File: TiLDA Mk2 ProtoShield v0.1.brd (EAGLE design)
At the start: 67.9 x 100 mm, 104 parts

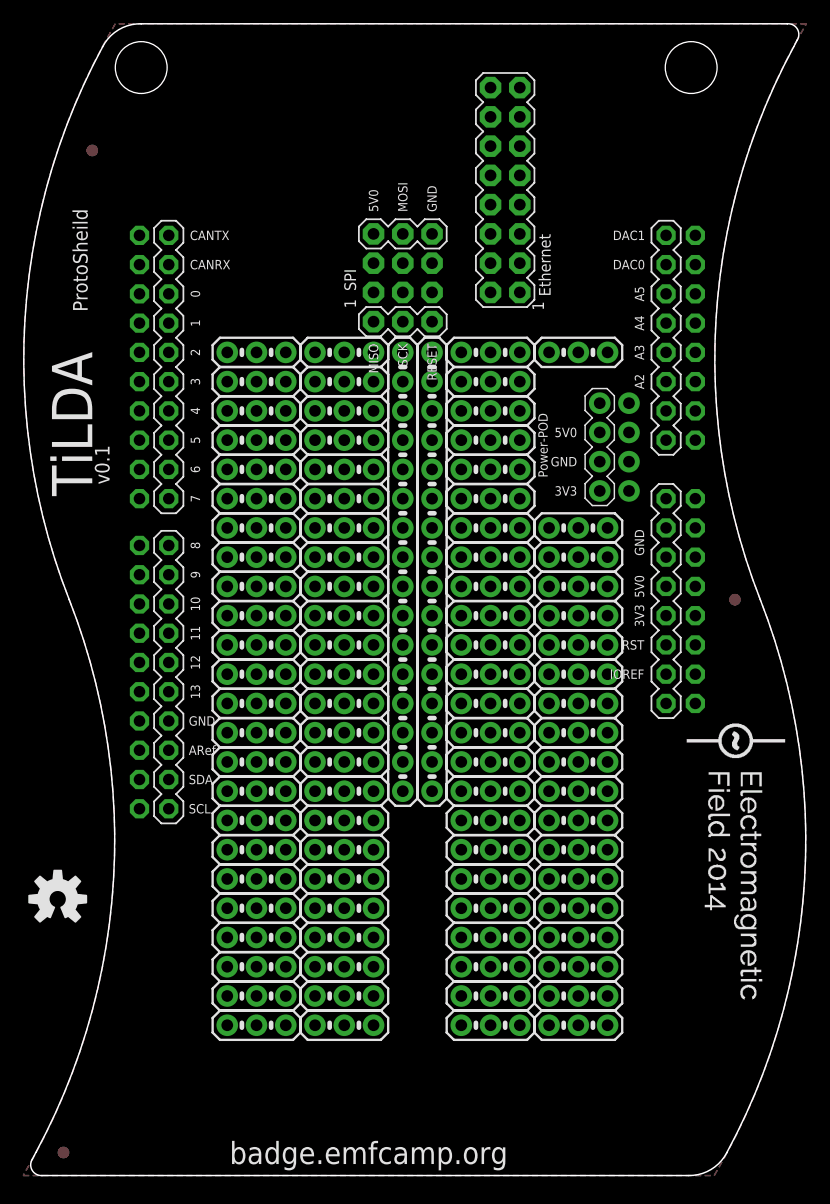
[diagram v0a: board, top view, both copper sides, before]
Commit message: ProtoShield: lots more work
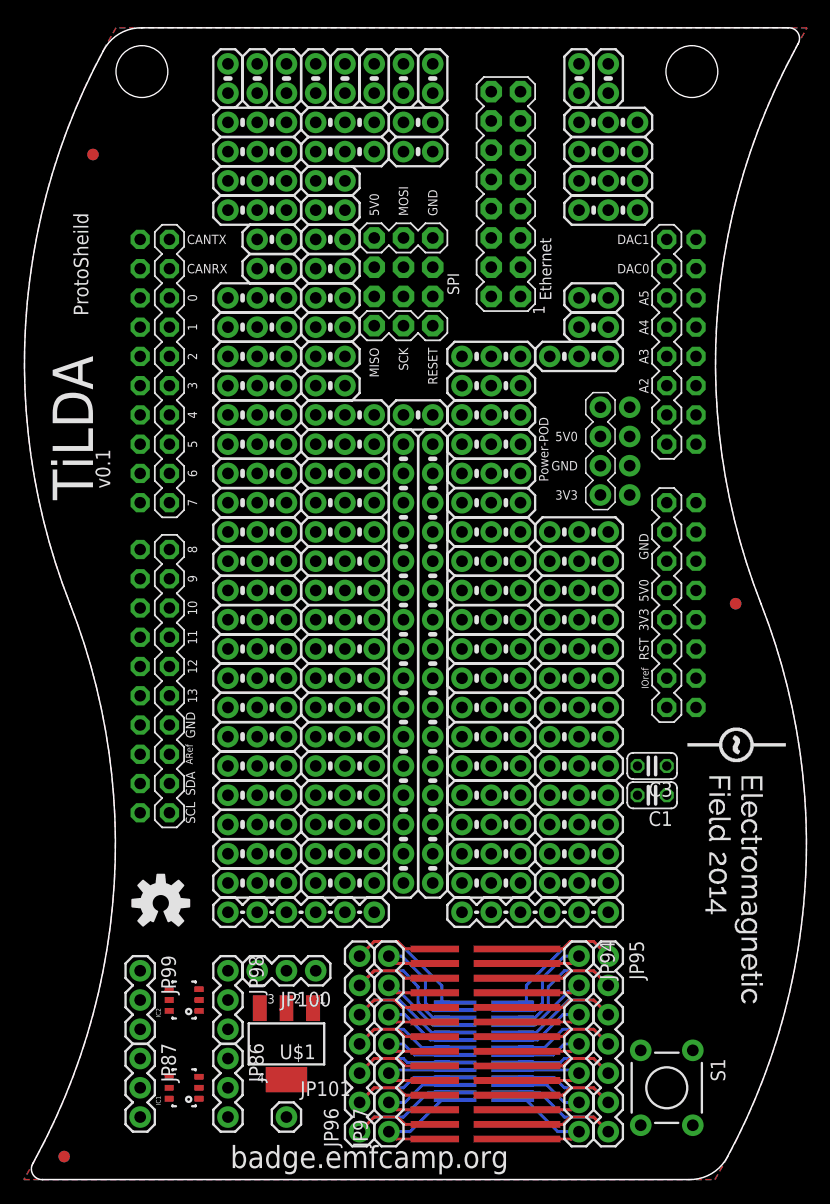
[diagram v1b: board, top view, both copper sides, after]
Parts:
- removed JP88, JP89, JP90, JP91, JP92, JP93: (no value), TiLDA Mk2 Parts:1X03_PROTO_SILK
- added C1, C3: 100nF, rcl:C025-024X044
- added IC1, IC2: SOT-23-6, TiLDA Mk2 Parts:SOT-23-6
- added JP100, JP98, JP99: (no value), TiLDA Mk2 Parts:1X03
- added JP101: M01PTH, TiLDA Mk2 Parts:1X01
- added JP102, JP103, JP104, JP105, JP106, JP107, JP108, JP109, JP110, JP111, JP112, JP113, JP114, JP115, JP116, JP117, JP118, JP119, JP120, JP121, JP122, JP123, JP124, JP125, JP126: (no value), TiLDA Mk2 Parts:1X02_PROTO_SILK
- added JP94, JP95, JP96, JP97: (no value), TiLDA Mk2 Parts:1X07
- added S1: (no value), CISECO eaglecad designs:TACTILE-PTH
- added U$1: TLV1117-33CDCY, TiLDA Mk2 Parts:SOT223
- added U$2: SSOP28-NOSLIK, CISECO eaglecad designs:SSOP28D-NOSILK
- added U$5: PICAXE-28X1-SO28-MULITWIDE, CISECO eaglecad designs:S028-MUTLIWIDE
- JP1, JP2: value M16PROTO_SILK -> (none)
- JP78, JP79: device TiLDA Mk2 Parts:1X03_PROTO_SILK -> TiLDA Mk2 Parts:1X06_PROTO_SLIK
- JP86, JP87: device TiLDA Mk2 Parts:1X03_PROTO_SILK -> TiLDA Mk2 Parts:1X03
- moved JP85 75.9 mm to (48.3, 91.4)
- moved JP69 74.4 mm to (48.3, 86.4)
- moved JP77 74.4 mm to (48.3, 83.8)
- moved JP84 74.0 mm to (48.3, 88.9)
- moved JP74 70.8 mm to (17.8, 88.9)
- moved JP75 70.8 mm to (25.4, 88.9)
- moved JP64 70.8 mm to (17.8, 91.4)
- moved JP67 70.8 mm to (25.4, 91.4)
- moved JP68 70.8 mm to (17.8, 86.4)
- moved JP76 70.8 mm to (17.8, 83.8)
- moved JP87 39.9 mm to (10.2, 10.2), turned to 270 degrees
- moved JP79 29.0 mm to (17.8, 22.9)
- moved JP86 27.2 mm to (17.8, 10.2), turned to 270 degrees
- moved JP72 20.5 mm to (38.1, 25.4)
- moved JP73 20.5 mm to (45.7, 25.4)
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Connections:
- removed net N$93: JP88.1, JP88.2, JP88.3
- removed net N$94: JP89.1, JP89.2, JP89.3
- removed net N$95: JP90.1, JP90.2, JP90.3
- removed net N$96: JP91.1, JP91.2, JP91.3
- removed net N$97: JP92.1, JP92.2, JP92.3
- removed net N$98: JP93.1, JP93.2, JP93.3
- new net N$100: IC1.4, JP87.1
- new net N$101: IC2.2, JP98.2
- new net N$102: IC2.1, JP98.3
- new net N$103: IC2.3, JP98.1
- new net N$104: IC2.5, JP99.2
- new net N$105: IC2.6, JP99.3
- new net N$106: IC2.4, JP99.1
- new net N$107: JP100.1, U$1.1
- new net N$108: JP100.2, U$1.2
- new net N$109: JP100.3, U$1.3
- new net N$110: JP101.1, U$1.4
- new net N$111: JP102.1, JP102.2
- new net N$112: JP103.1, JP103.2
- new net N$113: JP104.1, JP104.2
- new net N$114: JP105.1, JP105.2
- new net N$115: JP106.1, JP106.2
- new net N$116: JP107.1, JP107.2
- new net N$117: JP108.1, JP108.2
- new net N$118: JP109.1, JP109.2
- new net N$119: JP110.1, JP110.2
- new net N$120: JP111.1, JP111.2
- new net N$121: JP112.1, JP112.2
- new net N$122: JP113.1, JP113.2
- new net N$123: JP114.1, JP114.2
- new net N$124: JP115.1, JP115.2
- new net N$125: JP116.1, JP116.2
- new net N$126: JP117.1, JP117.2
- new net N$127: JP118.1, JP118.2
- new net N$128: JP119.1, JP119.2
- new net N$129: JP120.1, JP120.2
- new net N$130: JP121.1, JP121.2
- new net N$131: JP122.1, JP122.2
- new net N$132: JP123.1, JP123.2
- new net N$133: JP124.1, JP124.2
- new net N$134: JP125.1, JP125.2
- new net N$136: JP126.1, JP126.2
- new net N$99: IC1.6, JP87.3
- new net S1: JP94.7, U$2.28, U$5.1
- new net S10: JP95.3, U$2.19, U$5.10
- new net S11: JP94.2, U$2.18, U$5.11
- new net S12: JP95.2, U$2.17, U$5.12
- new net S13: JP94.1, U$2.16, U$5.13
- new net S14: JP95.1, U$2.15, U$5.14
- new net S15: JP96.7, U$2.14, U$5.15
- new net S16: JP97.7, U$2.13, U$5.16
- new net S17: JP96.6, U$2.12, U$5.17
- new net S18: JP97.6, U$2.11, U$5.18
- new net S19: JP96.5, U$2.10, U$5.19
- new net S2: JP95.7, U$2.27, U$5.2
- new net S20: JP97.5, U$2.9, U$5.20
- new net S21: JP96.4, U$2.8, U$5.21
- new net S22: JP97.4, U$2.7, U$5.22
- new net S23: JP96.3, U$2.6, U$5.23
- new net S24: JP97.3, U$2.5, U$5.24
- new net S25: JP96.2, U$2.4, U$5.25
- new net S26: JP97.2, U$2.3, U$5.26
- new net S27: JP96.1, U$2.2, U$5.27
- new net S28: JP97.1, U$2.1, U$5.28
- new net S3: JP94.6, U$2.26, U$5.3
- new net S32: JP95.6, U$2.25, U$5.4
- new net S5: JP94.5, U$2.24, U$5.5
- new net S6: JP95.5, U$2.23, U$5.6
- new net S7: JP94.4, U$2.22, U$5.7
- new net S8: JP95.4, U$2.21, U$5.8
- new net S9: JP94.3, U$2.20, U$5.9
- net !RESET: now also S1.3
- net 3V3: now also C1.2
- net 5V0: now also C3.2
- net GND: now also C1.1, C3.1, S1.1
- net N$1: now also JP79.1, JP79.2, JP79.3, JP79.4, JP79.5, JP79.6
- net N$2: now also JP78.1, JP78.2, JP78.3, JP78.4, JP78.5, JP78.6
- net N$83: now also IC1.2, JP86.2; no longer JP78.1, JP78.2, JP78.3
- net N$84: now also IC1.1, JP86.3; no longer JP79.1, JP79.2, JP79.3
- net N$91: now also IC1.3; no longer JP86.2, JP86.3
- net N$92: now also IC1.5; no longer JP87.1, JP87.3
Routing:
- net S14: track 0.00 -> 19.6 mm
- net S12: track 0.00 -> 19.0 mm
- net S15: track 0.00 -> 18.0 mm
- net S10: track 0.00 -> 17.6 mm
- net S17: track 0.00 -> 17.5 mm
- net S2: track 0.00 -> 17.3 mm
- net S8: track 0.00 -> 17.0 mm
- net S32: track 0.00 -> 16.8 mm
- net S6: track 0.00 -> 16.5 mm
- net S19: track 0.00 -> 16.2 mm
- net S27: track 0.00 -> 15.9 mm
- net S21: track 0.00 -> 15.6 mm
- net S25: track 0.00 -> 15.4 mm
- net S23: track 0.00 -> 15.1 mm
- net S13: track 0.00 -> 13.5 mm
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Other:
- board text added: "-0.06, 0.35"
